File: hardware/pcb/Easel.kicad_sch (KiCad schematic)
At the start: 10 parts, among them J1 TFT2.8", K1 KEYSW, K2 KEYSW, K3 KEYSW, K4 KEYSW, U1 PicoW

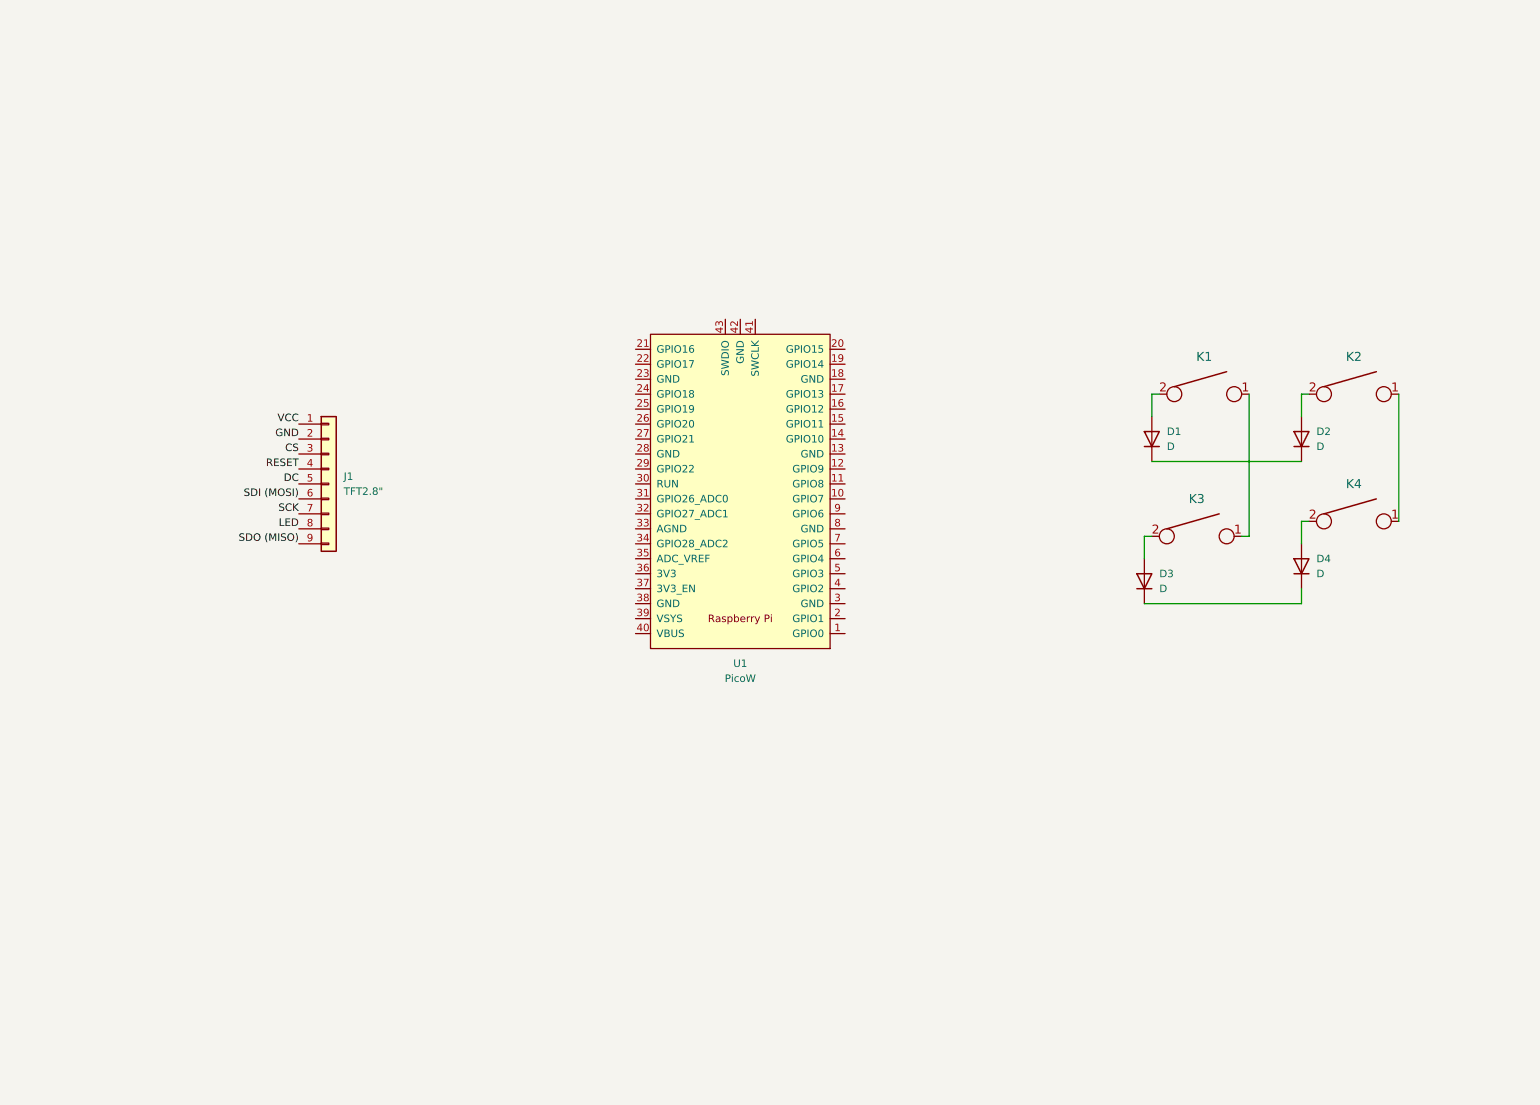
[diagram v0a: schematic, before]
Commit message: Update README
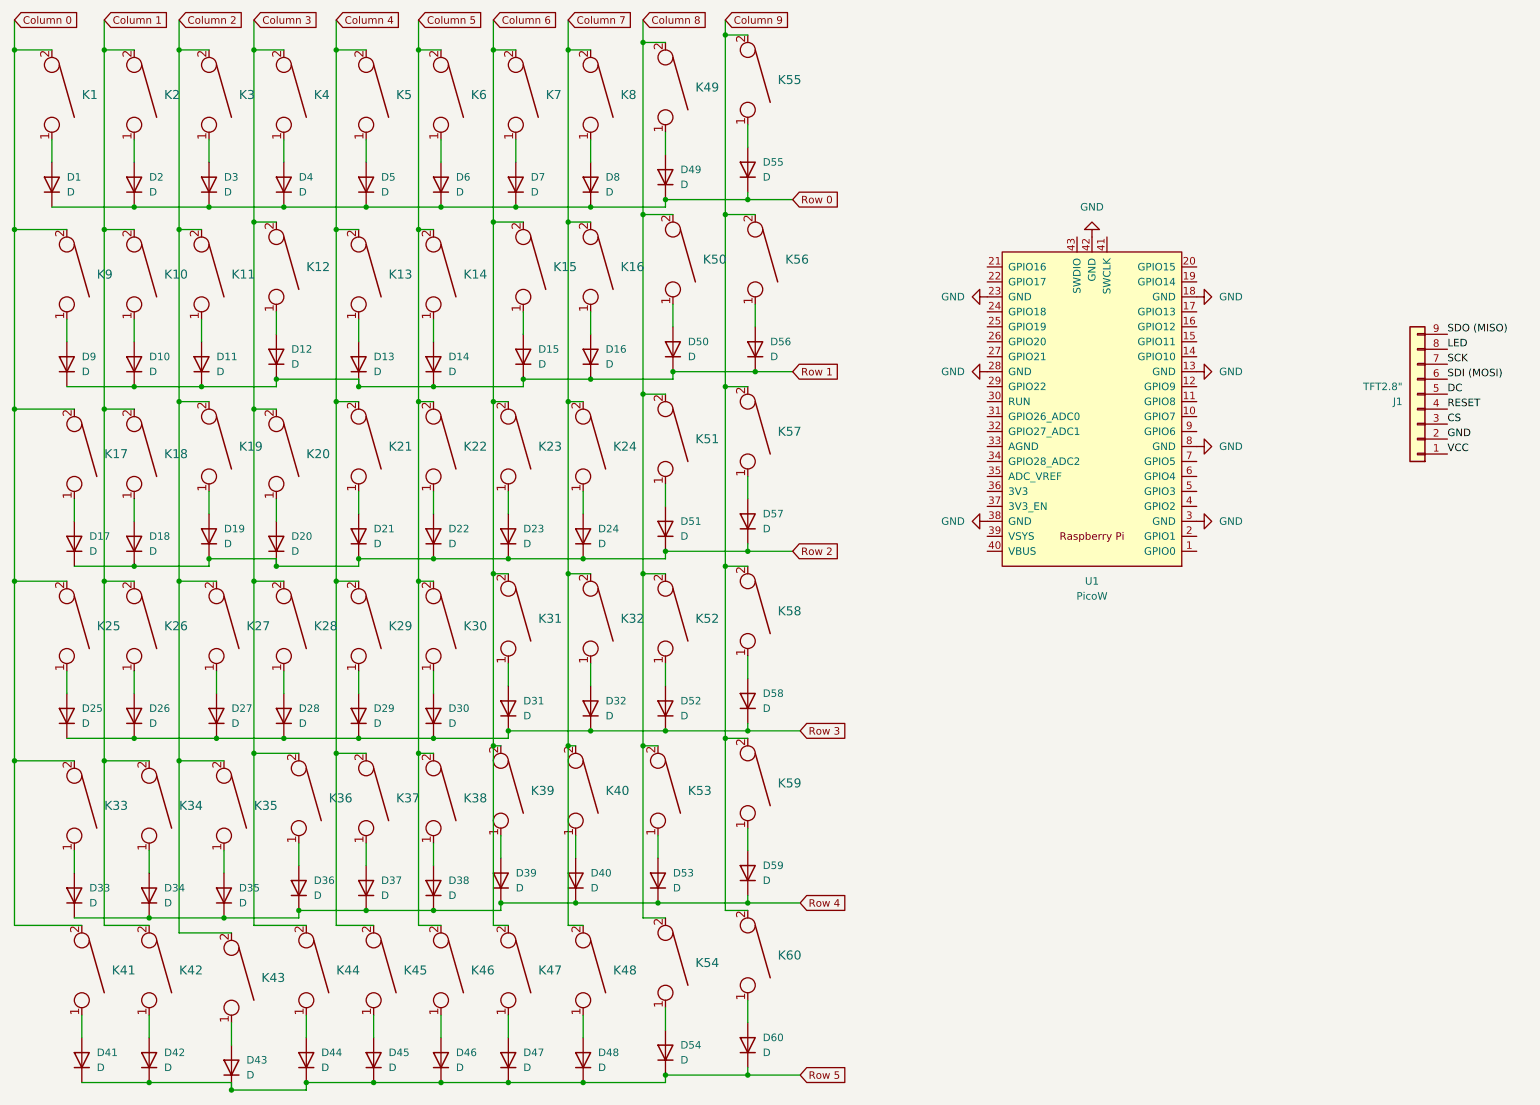
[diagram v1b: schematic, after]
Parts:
- added D10, D11, D12, D13, D14, D15, D16, D17, D18, D19, D20, D21, D22, D23, D24, D25, D26, D27, D28, D29, D30, D31, D32, D33, D34, D35, D36, D37, D38, D39, D40, D41, D42, D43, D44, D45, D46, D47, D48, D49, D5, D50, D51, D52, D53, D54, D55, D56, D57, D58, D59, D6, D60, D7, D8, D9: D, symbol Device:D
- added K10, K11, K12, K13, K14, K15, K16, K17, K18, K19, K20, K21, K22, K23, K24, K25, K26, K27, K28, K29, K30, K31, K32, K33, K34, K35, K36, K37, K38, K39, K40, K41, K42, K43, K44, K45, K46, K47, K48, K49, K5, K50, K51, K52, K53, K54, K55, K56, K57, K58, K59, K6, K60, K7, K8, K9: KEYSW, symbol keyboard_parts:KEYSW
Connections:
- net GND: now also U1.13 (GND), U1.18 (GND), U1.23 (GND), U1.28 (GND), U1.3 (GND), U1.38 (GND), U1.42 (GND), U1.8 (GND)
- net at K1.1: now also D1.2 (A); no longer K3.1
- net Column 0: now reaches K1.2
- net Column 0: now also K17.2, K25.2, K33.2, K41.2, K9.2; no longer D1.2 (A)
- net at K4.1: now also D4.2 (A); no longer K2.1
- net at D2.2 (A): now also K2.1; no longer K2.2
- net Row 0: now reaches D1.1 (K), D2.1 (K)
- net Row 0: now also D3.1 (K), D4.1 (K), D49.1 (K), D5.1 (K), D55.1 (K), D6.1 (K), D7.1 (K), D8.1 (K)
- net Column 3: now reaches K4.2
- net Column 3: now also K12.2, K20.2, K28.2, K36.2, K44.2; no longer D4.2 (A)
- net at D3.2 (A): now also K3.1; no longer K3.2
- new net: D20.2 (A), K20.1
- new net: D51.2 (A), K51.1
- new net: D38.2 (A), K38.1
- new net: D7.2 (A), K7.1
- new net: D59.2 (A), K59.1
- new net: D37.2 (A), K37.1
- new net: D35.2 (A), K35.1
- new net: D52.2 (A), K52.1
- new net: D26.2 (A), K26.1
- new net: D34.2 (A), K34.1
- new net: D50.2 (A), K50.1
- new net: D21.2 (A), K21.1
- new net: D48.2 (A), K48.1
- new net: D15.2 (A), K15.1
- new net: D13.2 (A), K13.1
- new net: D40.2 (A), K40.1
- new net: D53.2 (A), K53.1
- new net: D58.2 (A), K58.1
- new net: D57.2 (A), K57.1
- new net: D32.2 (A), K32.1
- new net: D11.2 (A), K11.1
- new net: D18.2 (A), K18.1
- new net: D22.2 (A), K22.1
- new net: D25.2 (A), K25.1
- new net: D24.2 (A), K24.1
- new net: D8.2 (A), K8.1
- new net: D23.2 (A), K23.1
- new net: D5.2 (A), K5.1
- new net: D19.2 (A), K19.1
- new net: D9.2 (A), K9.1
- new net: D16.2 (A), K16.1
- new net: D39.2 (A), K39.1
- new net: D47.2 (A), K47.1
- new net: D28.2 (A), K28.1
- new net: D54.2 (A), K54.1
- new net: D14.2 (A), K14.1
- new net: D29.2 (A), K29.1
- new net: D12.2 (A), K12.1
- new net: D31.2 (A), K31.1
- new net: D43.2 (A), K43.1
- new net: D6.2 (A), K6.1
- new net: D49.2 (A), K49.1
- new net: D30.2 (A), K30.1
- new net: D45.2 (A), K45.1
- new net: D10.2 (A), K10.1
- new net: D46.2 (A), K46.1
- new net: D27.2 (A), K27.1
- new net: D42.2 (A), K42.1
- new net: D17.2 (A), K17.1
- new net: D60.2 (A), K60.1
- new net: D36.2 (A), K36.1
- new net: D33.2 (A), K33.1
- new net: D56.2 (A), K56.1
- new net: D44.2 (A), K44.1
- new net: D55.2 (A), K55.1
- new net: D41.2 (A), K41.1
- new net Column 1: K10.2, K18.2, K2.2, K26.2, K34.2, K42.2
- new net Column 2: K11.2, K19.2, K27.2, K3.2, K35.2, K43.2
- new net Column 4: K13.2, K21.2, K29.2, K37.2, K45.2, K5.2
- new net Column 5: K14.2, K22.2, K30.2, K38.2, K46.2, K6.2
- new net Column 6: K15.2, K23.2, K31.2, K39.2, K47.2, K7.2
- new net Column 7: K16.2, K24.2, K32.2, K40.2, K48.2, K8.2
- new net Column 8: K49.2, K50.2, K51.2, K52.2, K53.2, K54.2
- new net Column 9: K55.2, K56.2, K57.2, K58.2, K59.2, K60.2
- new net Row 1: D10.1 (K), D11.1 (K), D12.1 (K), D13.1 (K), D14.1 (K), D15.1 (K), D16.1 (K), D50.1 (K), D56.1 (K), D9.1 (K)
- new net Row 2: D17.1 (K), D18.1 (K), D19.1 (K), D20.1 (K), D21.1 (K), D22.1 (K), D23.1 (K), D24.1 (K), D51.1 (K), D57.1 (K)
- new net Row 3: D25.1 (K), D26.1 (K), D27.1 (K), D28.1 (K), D29.1 (K), D30.1 (K), D31.1 (K), D32.1 (K), D52.1 (K), D58.1 (K)
- new net Row 4: D33.1 (K), D34.1 (K), D35.1 (K), D36.1 (K), D37.1 (K), D38.1 (K), D39.1 (K), D40.1 (K), D53.1 (K), D59.1 (K)
- new net Row 5: D41.1 (K), D42.1 (K), D43.1 (K), D44.1 (K), D45.1 (K), D46.1 (K), D47.1 (K), D48.1 (K), D54.1 (K), D60.1 (K)
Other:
- moved on the sheet: J1, U1
